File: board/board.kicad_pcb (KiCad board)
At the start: 2 copper layers, 21 x 13 mm, 1 part

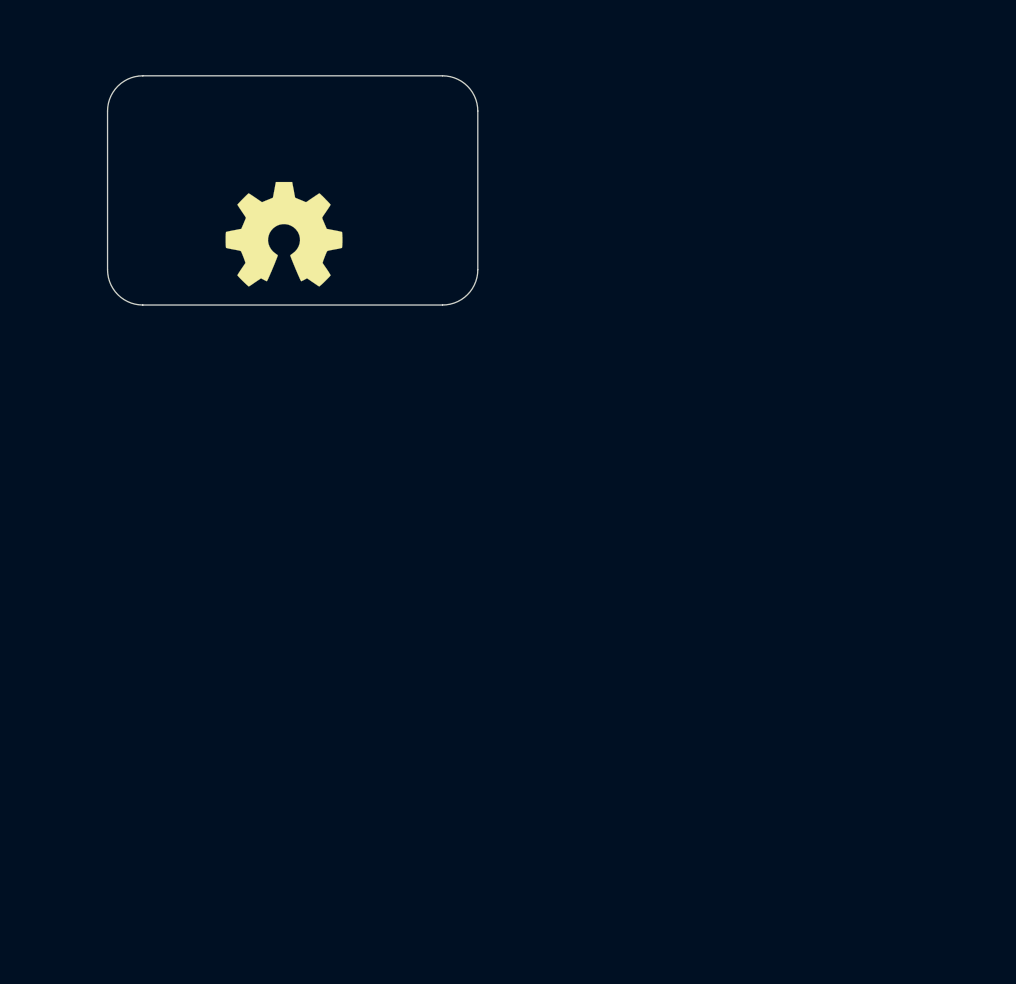
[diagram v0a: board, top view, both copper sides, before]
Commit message: initial
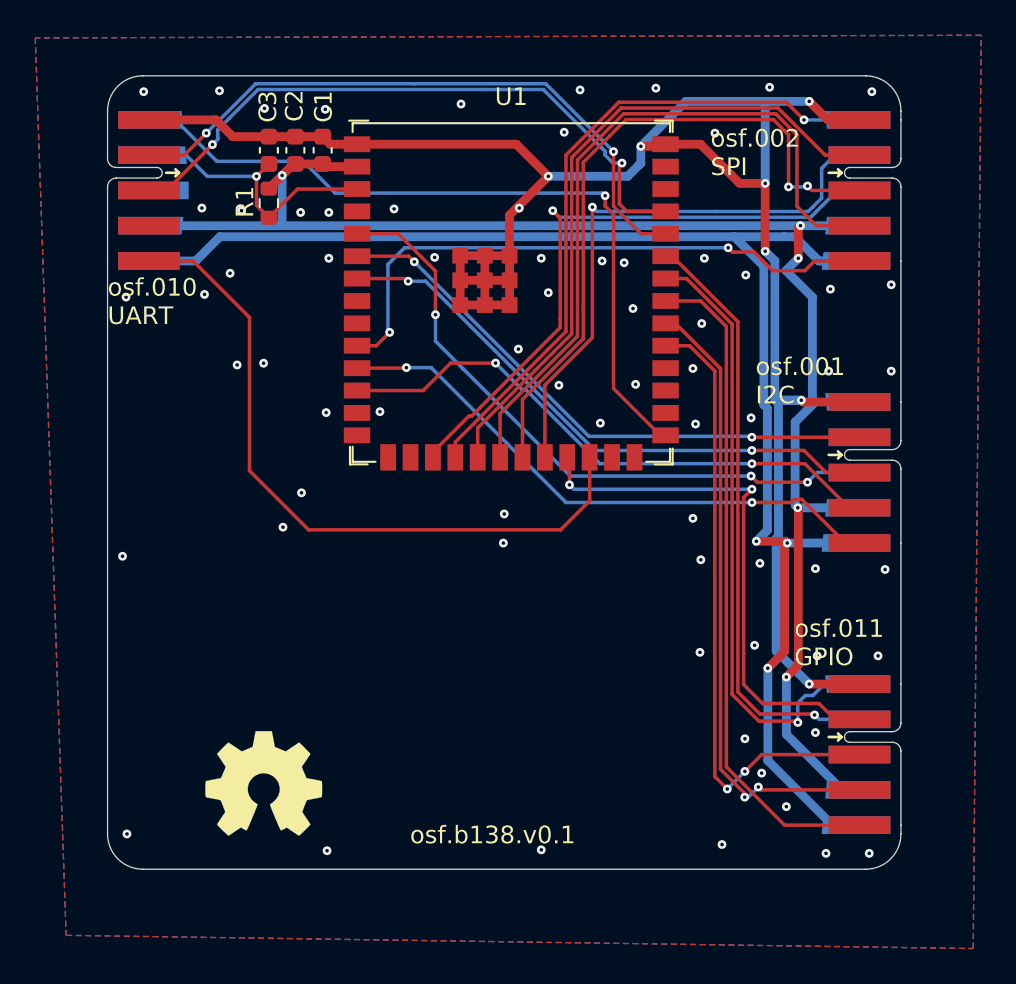
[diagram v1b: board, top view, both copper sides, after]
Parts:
- added C1: 1uF, Capacitor_SMD:C_0603_1608Metric, F.Cu at (152.2, 94.2)
- added C2: 10uF, Capacitor_SMD:C_0603_1608Metric, F.Cu at (150.7, 94.2)
- added C3: 1uF, Capacitor_SMD:C_0603_1608Metric, F.Cu at (149.2, 94.2)
- added J1: 010_UART, on_edge:on_edge_2x05_device, F.Cu at (140.0, 96.5)
- added J2: 002_SPI, on_edge:on_edge_2x05_host, F.Cu at (185.0, 96.5)
- added J3: 011_GPIO, on_edge:on_edge_2x05_host, F.Cu at (185.0, 128.5)
- added J4: 001_I2C, on_edge:on_edge_2x05_host, F.Cu at (185.0, 112.5)
- added R1: 10k, Resistor_SMD:R_0603_1608Metric, F.Cu at (149.2, 97.2)
- added U1: ESP32-S3-WROOM-1, b138:ESP32-S3-WROOM-1U, F.Cu at (162.9, 102.1)
- moved LOGO1 31.2 mm to (148.8, 130.2)
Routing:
- net GND: track 0.00 -> 117.8 mm, vias 0 -> 76
- net +3.3V: track 0.00 -> 88.1 mm, vias 0 -> 5
- net +5V: track 0.00 -> 84.7 mm, vias 0 -> 3
- net /esp/BOOT: track 0.00 -> 42.8 mm, vias 0 -> 1
- net /esp/SPI2_SCLK: track 0.00 -> 40.8 mm
- net /esp/U0_INT: track 0.00 -> 39.6 mm
- net /esp/SPI2_MISO: track 0.00 -> 38.3 mm, vias 0 -> 2
- net /esp/SPI2_CS: track 0.00 -> 38.0 mm, vias 0 -> 1
- net /esp/IO3: track 0.00 -> 37.9 mm
- net /esp/SPI2_MOSI: track 0.00 -> 37.8 mm
- net /esp/I2C_reset: track 0.00 -> 36.9 mm, vias 0 -> 3
- net /esp/U0TXD: track 0.00 -> 36.5 mm, vias 0 -> 2
- net /esp/U0RXD: track 0.00 -> 36.3 mm, vias 0 -> 2
- net /esp/IO2: track 0.00 -> 35.9 mm, vias 0 -> 2
- net /esp/IO1: track 0.00 -> 35.7 mm, vias 0 -> 2
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- added copper zone on B.Cu, net GND
- added copper zone on F.Cu, net GND
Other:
- board size 21 x 13 mm -> 45 x 45 mm
- board text added: "osf.001 I2C"
- board text added: "osf.002 SPI"
- board text added: "osf.010 UART"
- board text added: "osf.011 GPIO"
- board text added: "osf.b138.v0.1"
